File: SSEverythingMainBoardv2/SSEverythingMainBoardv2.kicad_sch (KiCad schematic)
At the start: 67 parts, among them J1 CONN_06SILK_FEMALE_PTH, J2 CONN_06SILK_FEMALE_PTH, J4 Switch, J5 Conn_01x02, J6 Conn_01x05, J8 Conn_01x03, M1 Left MOTOR, M2 Right MOTOR, Q1 PBSS4160DS, Q2 PBSS4160DS, Q3 PBSS4160DS, Q4 PBSS4160DS, SW1 TACT_SW, U1 DFRobot_DC_Controller

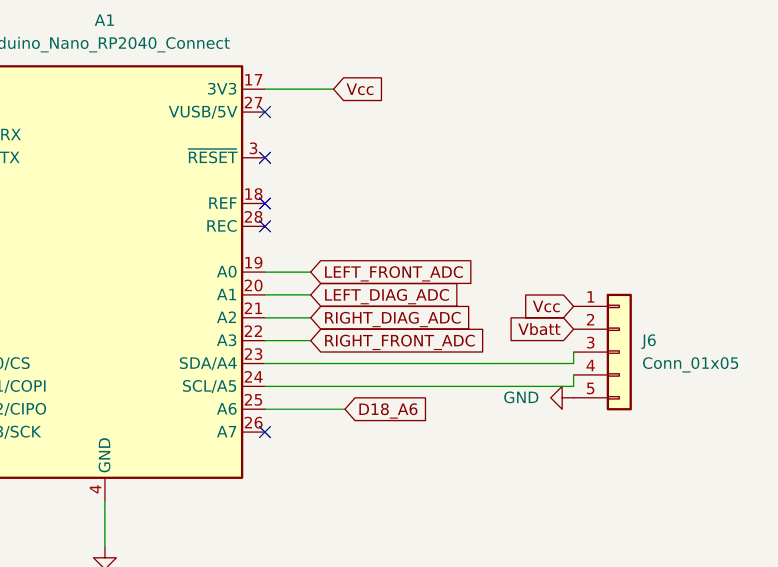
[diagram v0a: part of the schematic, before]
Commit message: routing changes
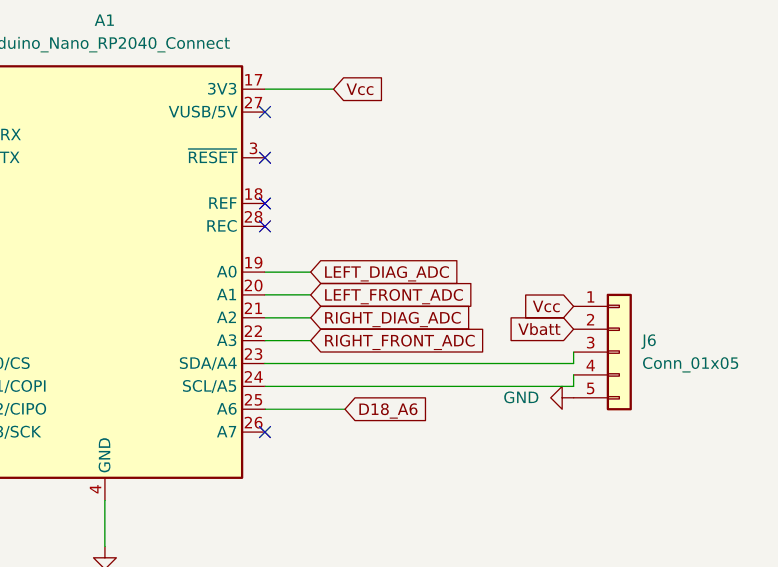
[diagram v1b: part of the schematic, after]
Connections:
- net LEFT_DIAG_ADC: now also A1.19 (A0); no longer A1.20 (A1)
- net LEFT_FRONT_ADC: now also A1.20 (A1); no longer A1.19 (A0)
